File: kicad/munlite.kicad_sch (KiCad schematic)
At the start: 19 parts, among them J1 Conn_Pover, J2 Conn_Pir, J3 Conn_Prog, J4 Conn_Opto, J5 Conn_Led, SW1 SW_Push, U1 STM32L031F6Px, U2 AP2112K-3.3, U3 CN5711

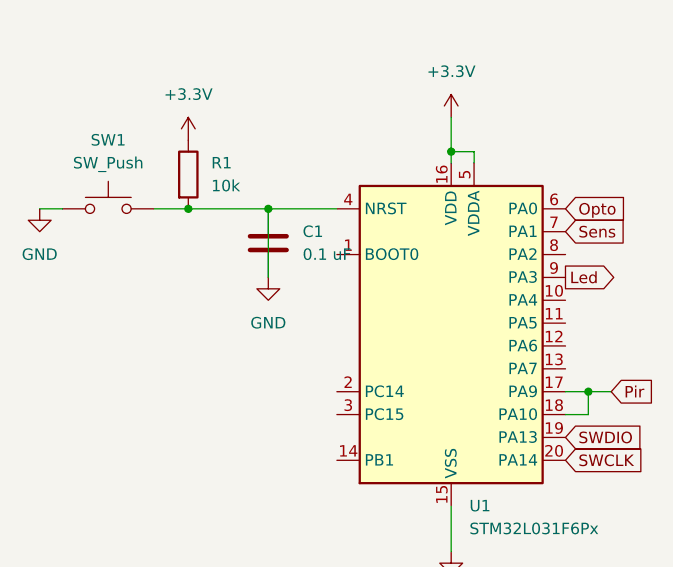
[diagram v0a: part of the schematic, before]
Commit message: kicad: update pcb
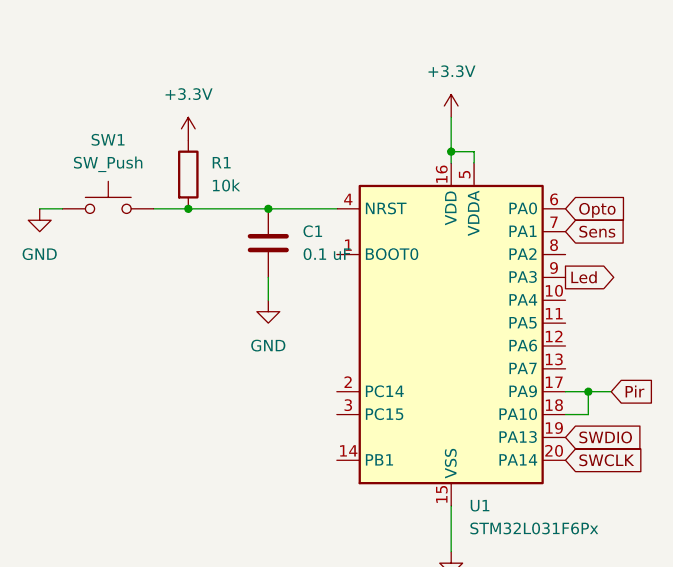
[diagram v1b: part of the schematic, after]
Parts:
- C1, C5, C6: footprint Capacitor_SMD:C_0805_2012Metric -> Capacitor_SMD:C_1206_3216Metric
- C4: footprint Capacitor_SMD:C_1210_3225Metric -> Capacitor_SMD:C_1206_3216Metric
- R1: footprint Resistor_SMD:R_0805_2012Metric -> Resistor_SMD:R_1206_3216Metric
- SW1: footprint Button_Switch_SMD:SW_SPST_EVQP2 -> Button_Switch_THT:SW_PUSH_6mm
- U1: footprint Package_SO:TSSOP-20_4.4x6.5mm_P0.65mm -> Connector_PinHeader_2.54mm:tssop20_adapter
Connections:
- net GND: no longer C1.1, R1.2, SW1.2, U1.4 (NRST)
- new net: C1.1, R1.2, SW1.2, U1.4 (NRST)
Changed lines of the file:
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@@
-    (stroke (width 0) (type default) (color 0 0 0 0))
-  )
-  (wire (pts (xy 52.07 74.93) (xy 52.07 67.31))
     (stroke (width 0) (type default) (color 0 0 0 0))
   )
@@
   )
   (wire (pts (xy 124.46 147.32) (xy 127.635 147.32))
+    (stroke (width 0) (type default) (color 0 0 0 0))
+  )
+  (wire (pts (xy 52.07 77.47) (xy 52.07 74.93))
     (stroke (width 0) (type default) (color 0 0 0 0))
   )
@@
       (effects (font (size 1.27 1.27)) (justify left))
     )
-    (property "Footprint" "Capacitor_SMD:C_0805_2012Metric" (id 2) (at 53.0352 74.93 0)
+    (property "Footprint" "Capacitor_SMD:C_1206_3216Metric" (id 2) (at 53.0352 74.93 0)
       (effects (font (size 1.27 1.27)) hide)
     )
@@
       (effects (font (size 1.27 1.27)) (justify left))
     )
-    (property "Footprint" "Package_SO:TSSOP-20_4.4x6.5mm_P0.65mm" (id 2) (at 62.23 97.79 0)
+    (property "Footprint" "Connector_PinHeader_2.54mm:tssop20_adapter" (id 2) (at 62.23 97.79 0)
       (effects (font (size 1.27 1.27)) (justify right) hide)
     )
@@
     (pin "1")
   )
-  (symbol (lib_id "power:GND") (at 52.07 74.93 0) (unit 1)
-    (in_bom yes) (on_board yes) (fields_autoplaced)
-    (property "Reference" "#PWR03" (id 0) (at 52.07 81.28 0)
-      (effects (font (size 1.27 1.27)) hide)
-    )
-    (property "Value" "GND" (id 1) (at 52.07 80.01 0))
-    (property "Footprint" "" (id 2) (at 52.07 74.93 0)
-      (effects (font (size 1.27 1.27)) hide)
-    )
-    (property "Datasheet" "" (id 3) (at 52.07 74.93 0)
+  (symbol (lib_id "power:GND") (at 52.07 77.47 0) (unit 1)
+    (in_bom yes) (on_board yes) (fields_autoplaced)
+    (property "Reference" "#PWR03" (id 0) (at 52.07 83.82 0)
+      (effects (font (size 1.27 1.27)) hide)
+    )
+    (property "Value" "GND" (id 1) (at 52.07 82.55 0))
+    (property "Footprint" "" (id 2) (at 52.07 77.47 0)
+      (effects (font (size 1.27 1.27)) hide)
+    )
+    (property "Datasheet" "" (id 3) (at 52.07 77.47 0)
       (effects (font (size 1.27 1.27)) hide)
     )
@@
       (effects (font (size 1.27 1.27)) (justify left))
     )
-    (property "Footprint" "Capacitor_SMD:C_0805_2012Metric" (id 2) (at 209.2452 29.21 0)
+    (property "Footprint" "Capacitor_SMD:C_1206_3216Metric" (id 2) (at 209.2452 29.21 0)
       (effects (font (size 1.27 1.27)) hide)
     )
@@
     (property "Reference" "SW1" (id 0) (at 34.29 59.69 0))
     (property "Value" "SW_Push" (id 1) (at 34.29 62.23 0))
-    (property "Footprint" "Button_Switch_SMD:SW_SPST_EVQP2" (id 2) (at 34.29 62.23 0)
+    (property "Footprint" "Button_Switch_THT:SW_PUSH_6mm" (id 2) (at 34.29 62.23 0)
       (effects (font (size 1.27 1.27)) hide)
     )
@@
       (effects (font (size 1.27 1.27)) (justify left))
     )
-    (property "Footprint" "Capacitor_SMD:C_0805_2012Metric" (id 2) (at 221.9452 29.21 0)
+    (property "Footprint" "Capacitor_SMD:C_1206_3216Metric" (id 2) (at 221.9452 29.21 0)
       (effects (font (size 1.27 1.27)) hide)
     )
@@
       (effects (font (size 1.27 1.27)) (justify left))
     )
-    (property "Footprint" "Resistor_SMD:R_0805_2012Metric" (id 2) (at 41.402 63.5 90)
+    (property "Footprint" "Resistor_SMD:R_1206_3216Metric" (id 2) (at 41.402 63.5 90)
       (effects (font (size 1.27 1.27)) hide)
     )
@@
       (effects (font (size 1.27 1.27)) (justify left))
     )
-    (property "Footprint" "Capacitor_SMD:C_1210_3225Metric" (id 2) (at 196.5452 29.21 0)
+    (property "Footprint" "Capacitor_SMD:C_1206_3216Metric" (id 2) (at 196.5452 29.21 0)
       (effects (font (size 1.27 1.27)) hide)
     )
@@
     )
     (path "/03c26c15-787f-4106-98a5-5f1ff2c3076f"
-      (reference "C1") (unit 1) (value "0.1 uF") (footprint "Capacitor_SMD:C_0805_2012Metric")
+      (reference "C1") (unit 1) (value "0.1 uF") (footprint "Capacitor_SMD:C_1206_3216Metric")
     )
     (path "/51830f66-18cf-4edb-b54e-530ef47f04e7"
@@
     )
     (path "/e9743a90-345e-43d4-8cc9-f2a4c7b6eb34"
-      (reference "C4") (unit 1) (value "10uF") (footprint "Capacitor_SMD:C_1210_3225Metric")
+      (reference "C4") (unit 1) (value "10uF") (footprint "Capacitor_SMD:C_1206_3216Metric")
     )
     (path "/2e1d8c86-d7fc-4157-be20-16fb3063fea3"
-      (reference "C5") (unit 1) (value "0.1uF") (footprint "Capacitor_SMD:C_0805_2012Metric")
+      (reference "C5") (unit 1) (value "0.1uF") (footprint "Capacitor_SMD:C_1206_3216Metric")
     )
     (path "/b65e54b3-e34d-4251-a6db-22a12230b6d4"
-      (reference "C6") (unit 1) (value "0.1uF") (footprint "Capacitor_SMD:C_0805_2012Metric")
+      (reference "C6") (unit 1) (value "0.1uF") (footprint "Capacitor_SMD:C_1206_3216Metric")
     )
     (path "/a7a6f83c-c6dd-4d7d-963f-a52343903fb8"
@@
     )
     (path "/bc8a2400-9ef4-46e2-a709-1a7c89abdf50"
-      (reference "R1") (unit 1) (value "10k") (footprint "Resistor_SMD:R_0805_2012Metric")
+      (reference "R1") (unit 1) (value "10k") (footprint "Resistor_SMD:R_1206_3216Metric")
     )
     (path "/025215b9-8ba8-4506-8b56-c21c90e6746b"
@@
     )
     (path "/8c23f299-6bff-4556-8b64-6b13a90c6c48"
-      (reference "SW1") (unit 1) (value "SW_Push") (footprint "Button_Switch_SMD:SW_SPST_EVQP2")
+      (reference "SW1") (unit 1) (value "SW_Push") (footprint "Button_Switch_THT:SW_PUSH_6mm")
     )
     (path "/051d4750-b73a-474f-abf5-a58dadb01c92"
-      (reference "U1") (unit 1) (value "STM32L031F6Px") (footprint "Package_SO:TSSOP-20_4.4x6.5mm_P0.65mm")
+      (reference "U1") (unit 1) (value "STM32L031F6Px") (footprint "Connector_PinHeader_2.54mm:tssop20_adapter")
     )
     (path "/a4b6769b-2ea8-4eae-a790-10e6230b809f"
